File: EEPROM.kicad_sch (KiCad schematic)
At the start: 22 parts, among them IC1 PCA6408APW, IC2 AT24CS01, U2 TPS613221ADBVT

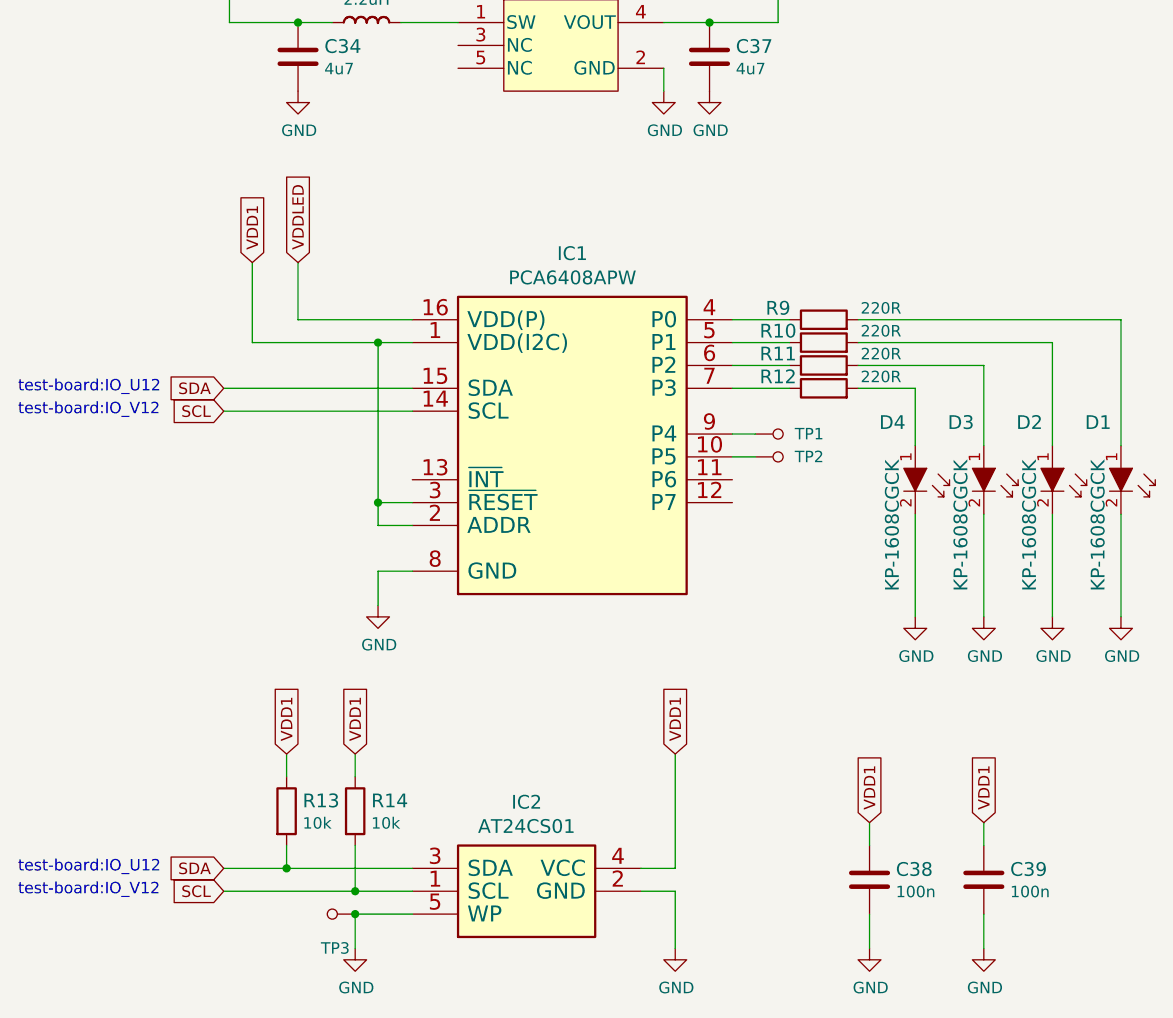
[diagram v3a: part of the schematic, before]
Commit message: Fix missing global links (wip), designators fixed
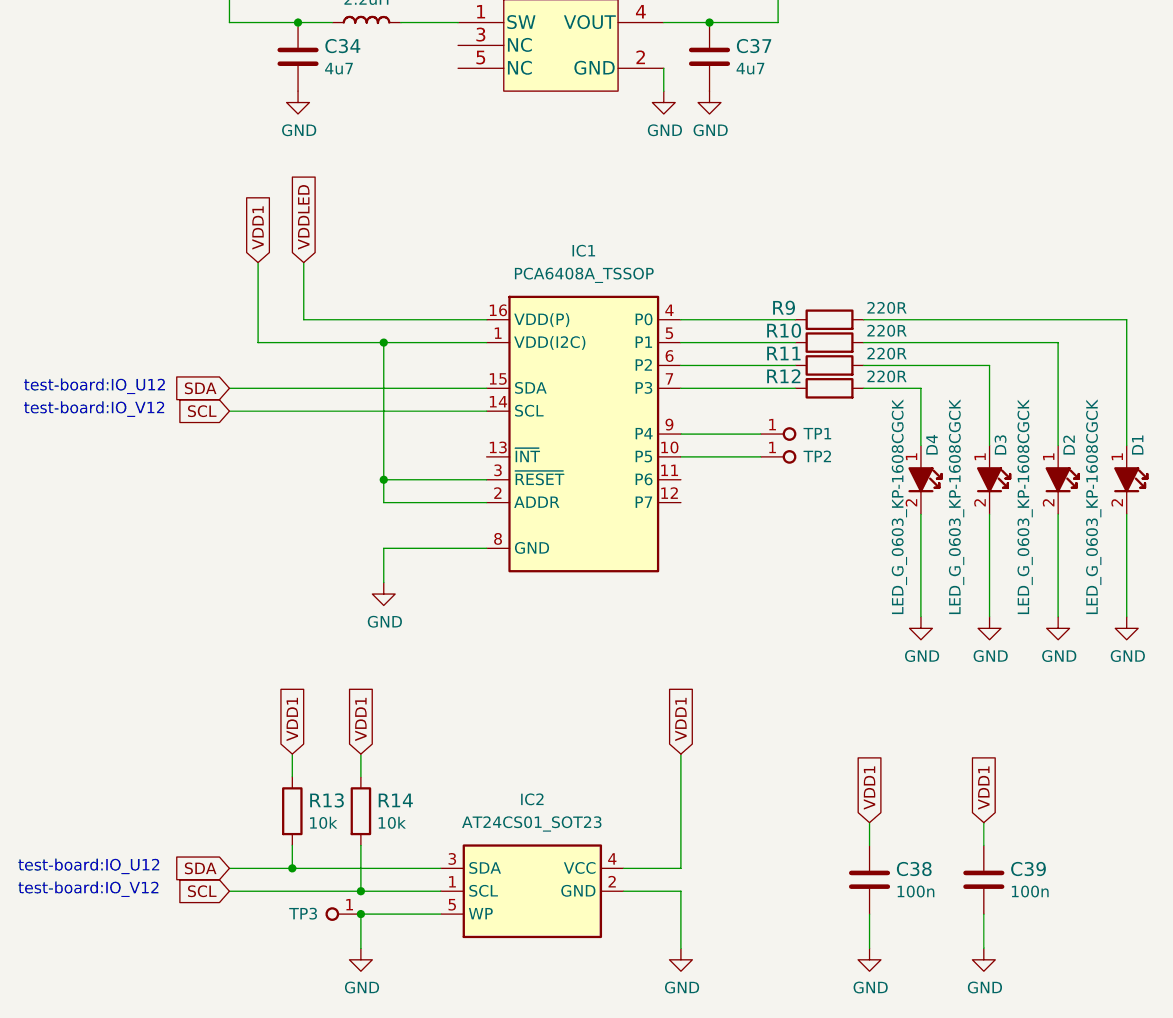
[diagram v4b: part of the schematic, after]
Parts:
- removed D1, D2, D3, D4: KP-1608CGCK, lpddr4-testbed-footprints:LED_0603, symbol lpddr4-testbed:KP-1608CGCK
- removed IC1: PCA6408APW, lpddr4-testbed-footprints:TSSOP-16, symbol lpddr4-testbed:PCA6408APW
- removed IC2: AT24CS01, lpddr4-testbed-footprints:SOT-23-5, symbol lpddr4-testbed:AT24CS01-antmicroMemory
- removed TP1, TP2, TP3: TP_SMD1MM, lpddr4-testbed-footprints:Testpoint_smd_1mm, symbol lpddr4-testbed:TP_SMD1MM
- added D1, D2, D3, D4: LED_G_0603_KP-1608CGCK, antmicro-footprints:LED_0603_1608Metric_G, symbol antmicroLEDIndicationDiscrete:LED_G_0603_KP-1608CGCK
- added IC1: PCA6408A_TSSOP, antmicro-footprints:TSSOP-16_4.4x5mm_P0.65mm, symbol antmicroInterfaceIOExpanders:PCA6408A_TSSOP
- added IC2: AT24CS01_SOT23, antmicro-footprints:SOT-23-5, symbol antmicroMemory:AT24CS01_SOT23
- added TP1, TP2, TP3: TP_0.75mm_SMD, antmicro-footprints:TP_SMD_0.75mm, symbol antmicroTestPoints:TP_0.75mm_SMD
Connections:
- net GND: now also D1.2, D2.2, D3.2, D4.2, IC1.8 (GND), IC2.2 (GND), IC2.5 (WP), TP3.1
- net SCL: now also IC1.14 (SCL), IC2.1 (SCL)
- net SDA: now also IC1.15 (SDA), IC2.3 (SDA)
- net VDD1: now also IC1.1 (VDD(I2C)), IC1.2 (ADDR), IC1.3 (~{RESET}), IC2.4 (VCC)
- net VDDLED: now also IC1.16 (VDD(P))
- net at R9.1: now also IC1.4 (P0)
- net at R9.2: now also D1.1
- net at R10.1: now also IC1.5 (P1)
- net at R10.2: now also D2.1
- net at R11.1: now also IC1.6 (P2)
- net at R11.2: now also D3.1
- net at R12.2: now also D4.1
- net at R12.1: now also IC1.7 (P3)
- new net: IC1.9 (P4), TP1.1
- new net: IC1.10 (P5), TP2.1
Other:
- moved on the sheet: R10, R11, R12, R13, R14, R9
